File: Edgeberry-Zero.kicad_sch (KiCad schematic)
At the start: 28 parts, among them J1 Molex_KK_1x02_P2.54mm, J2 Raspberry_Pi_2_3, J3 Edgeberry Cartridge Connector, P1 12Vin, Q1 BC547, Q2 BC547, Q3 BC547, SW1 SW_PUSH, U1 24LC256, U2 LM2596S-5.0

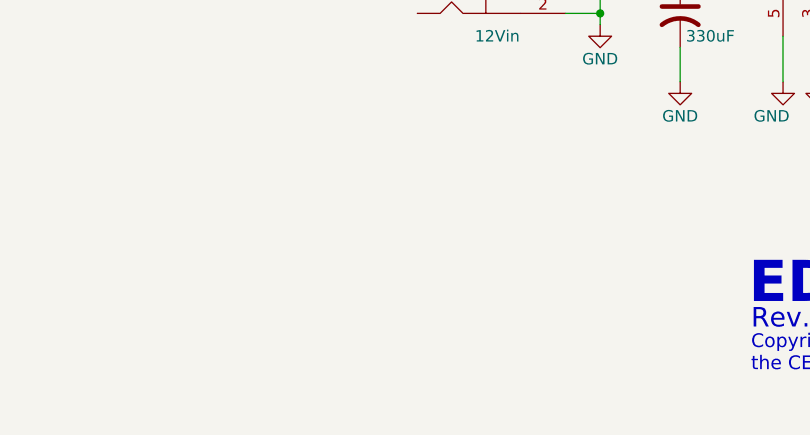
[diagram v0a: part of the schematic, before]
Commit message: Finished design
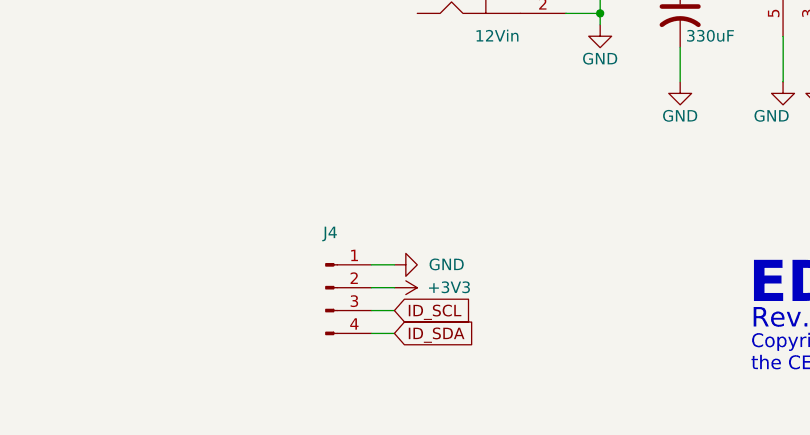
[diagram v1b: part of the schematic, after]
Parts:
- added J4: Conn_01x04_Pin, Connector_PinHeader_2.54mm:PinHeader_1x04_P2.54mm_Horizontal, symbol Connector:Conn_01x04_Pin
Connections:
- net +3V3: now also J4.2 (Pin_2)
- net GND: now also J4.1 (Pin_1)
- net ID_SCL: now also J4.3 (Pin_3)
- net ID_SDA: now also J4.4 (Pin_4)
